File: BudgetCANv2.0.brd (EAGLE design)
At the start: 24.4 x 46.4 mm, 34 parts, among them IC1 TJA1051T_3_CM,118, IC2 STM32G431C6T6, J2 USB4105-GF-A, J3 1776275-3, U2 AP2202K-3.3TRG1

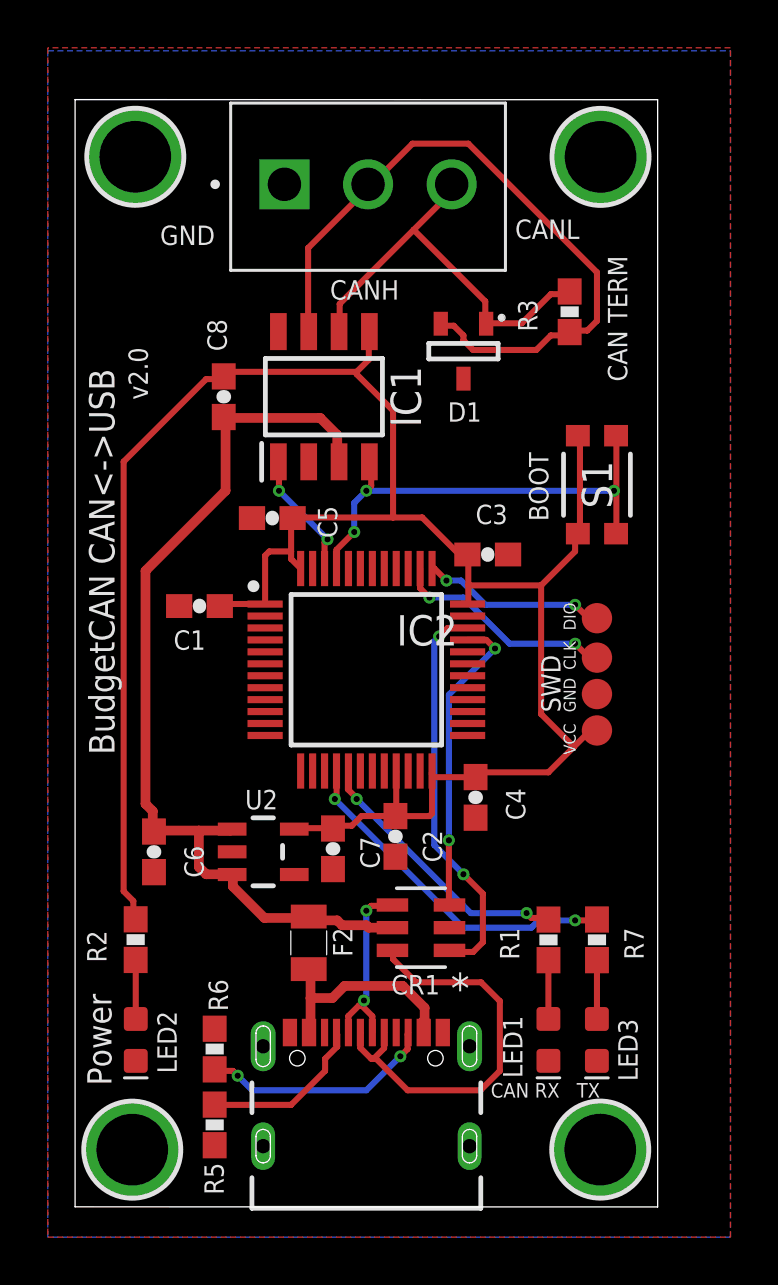
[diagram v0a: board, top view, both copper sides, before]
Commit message: Add files via upload
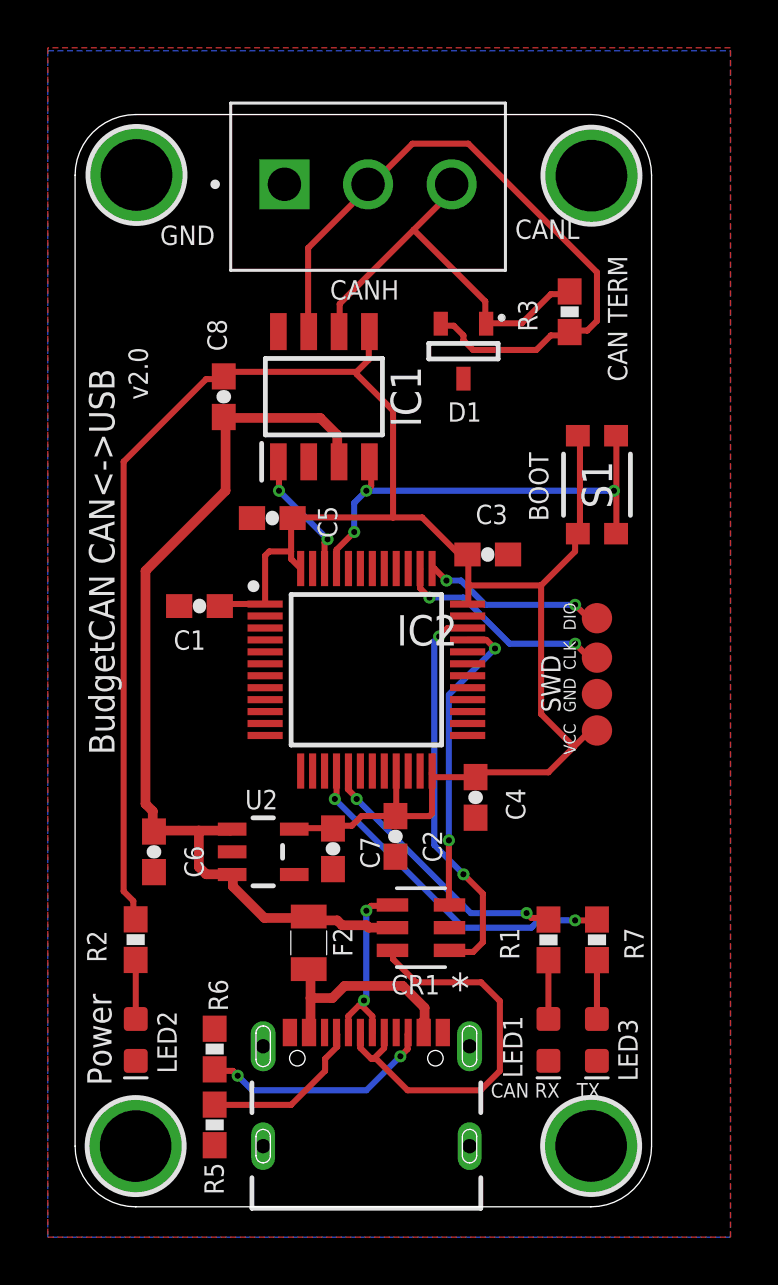
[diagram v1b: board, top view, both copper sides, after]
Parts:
- moved U$5 0.87 mm to (21.6, 43.2)
- moved U$4 0.76 mm to (2.57, 43.2)
- moved U$3 0.41 mm to (21.6, 2.55)
- moved U$2 0.21 mm to (2.53, 2.54)
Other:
- board size 24.4 x 46.4 mm -> 24.1 x 45.7 mm
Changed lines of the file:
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@@
 <setting verticaltext="up"/>
 </settings>
-<grid distance="5" unitdist="mil" unit="mil" style="lines" multiple="1" display="yes" altdistance="0.1" altunitdist="mil" altunit="mil"/>
+<grid distance="50" unitdist="mil" unit="mil" style="lines" multiple="1" display="yes" altdistance="1" altunitdist="mil" altunit="mil"/>
 <layers>
 <layer number="1" name="Top" color="4" fill="1" visible="yes" active="yes"/>
@@
 <board>
 <plain>
-<wire x1="0" y1="0" x2="24.3842" y2="-0.005078125" width="0" layer="20"/>
-<wire x1="24.3842" y1="-0.005078125" x2="24.3842" y2="46.339921875" width="0" layer="20"/>
-<wire x1="24.3842" y1="46.339921875" x2="0" y2="46.345" width="0" layer="20"/>
-<wire x1="0" y1="46.345" x2="0" y2="0" width="0" layer="20"/>
 <dimension x1="0" y1="46.345" x2="24.435" y2="46.345" x3="12.2175" y3="53.339996875" textsize="1.778" layer="20"/>
 <text x="19.812" y="28.702" size="0.8128" layer="21" rot="R90">BOOT</text>
@@
 <text x="10.541" y="33.782" size="1.778" layer="22" rot="MR270">Now with CANFD!</text>
 <dimension x1="0" y1="46.355" x2="0" y2="0" x3="-6.223" y3="23.1775" textsize="1.778" layer="20"/>
+<wire x1="0" y1="2.54" x2="2.54" y2="0" width="0" layer="20" curve="90"/>
+<wire x1="2.54" y1="0" x2="21.59" y2="0" width="0" layer="20"/>
+<wire x1="21.59" y1="0" x2="24.13" y2="2.54" width="0" layer="20" curve="90"/>
+<wire x1="24.13" y1="2.54" x2="24.13" y2="43.18" width="0" layer="20"/>
+<wire x1="24.13" y1="43.18" x2="21.59" y2="45.72" width="0" layer="20" curve="90"/>
+<wire x1="21.59" y1="45.72" x2="2.54" y2="45.72" width="0" layer="20"/>
+<wire x1="2.54" y1="45.72" x2="0" y2="43.18" width="0" layer="20" curve="90"/>
+<wire x1="0" y1="43.18" x2="0" y2="2.54" width="0" layer="20"/>
 </plain>
 <attributes>
@@
 <attribute name="VALUE" x="20.701" y="12.192" size="0.4064" layer="27" font="vector" rot="R270"/>
 </element>
-<element name="U$2" library="microbuilder" package="MOUNTINGHOLE_3.0_PLATEDTHIN" value="MOUNTINGHOLE3.0THIN" x="2.39268125" y="2.39268125" smashed="yes"/>
-<element name="U$3" library="microbuilder" package="MOUNTINGHOLE_3.0_PLATEDTHIN" value="MOUNTINGHOLE3.0THIN" x="21.981159375" y="2.39521875" smashed="yes"/>
-<element name="U$4" library="microbuilder" package="MOUNTINGHOLE_3.0_PLATEDTHIN" value="MOUNTINGHOLE3.0THIN" x="2.51968125" y="43.952159375" smashed="yes"/>
-<element name="U$5" library="microbuilder" package="MOUNTINGHOLE_3.0_PLATEDTHIN" value="MOUNTINGHOLE3.0THIN" x="21.993859375" y="43.947078125" smashed="yes"/>
+<element name="U$2" library="microbuilder" package="MOUNTINGHOLE_3.0_PLATEDTHIN" value="MOUNTINGHOLE3.0THIN" x="2.534921875" y="2.542540625" smashed="yes"/>
+<element name="U$3" library="microbuilder" package="MOUNTINGHOLE_3.0_PLATEDTHIN" value="MOUNTINGHOLE3.0THIN" x="21.600159375" y="2.54761875" smashed="yes"/>
+<element name="U$4" library="microbuilder" package="MOUNTINGHOLE_3.0_PLATEDTHIN" value="MOUNTINGHOLE3.0THIN" x="2.57048125" y="43.190159375" smashed="yes"/>
+<element name="U$5" library="microbuilder" package="MOUNTINGHOLE_3.0_PLATEDTHIN" value="MOUNTINGHOLE3.0THIN" x="21.612859375" y="43.159678125" smashed="yes"/>
 <element name="TP1" library="SparkFun-Connectors" library_urn="urn:adsk.eagle:library:513" package="PAD.03X.05" package3d_urn="urn:adsk.eagle:package:38285/1" value="TEST-POINT3X5" x="21.844" y="19.939" smashed="yes"/>
 <element name="TP2" library="SparkFun-Connectors" library_urn="urn:adsk.eagle:library:513" package="PAD.03X.05" package3d_urn="urn:adsk.eagle:package:38285/1" value="TEST-POINT3X5" x="21.844" y="21.463" smashed="yes"/>
